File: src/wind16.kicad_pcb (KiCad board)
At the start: 2 copper layers, 78 x 78 mm, 49 parts, among them SW1 SW_Push_45deg, SW10 SW_Push_45deg, SW11 SW_Push_45deg, SW12 SW_Push_45deg, SW13 SW_Push_45deg, SW14 SW_Push_45deg, SW15 SW_Push_45deg, SW16 SW_Push_45deg, SW2 SW_Push_45deg, SW3 SW_Push_45deg, SW4 SW_Push_45deg, SW5 SW_Push_45deg, SW6 SW_Push_45deg, SW7 SW_Push_45deg, SW8 SW_Push_45deg, SW9 SW_Push_45deg, U1 MCU_Seeed_XIAO_RP2040

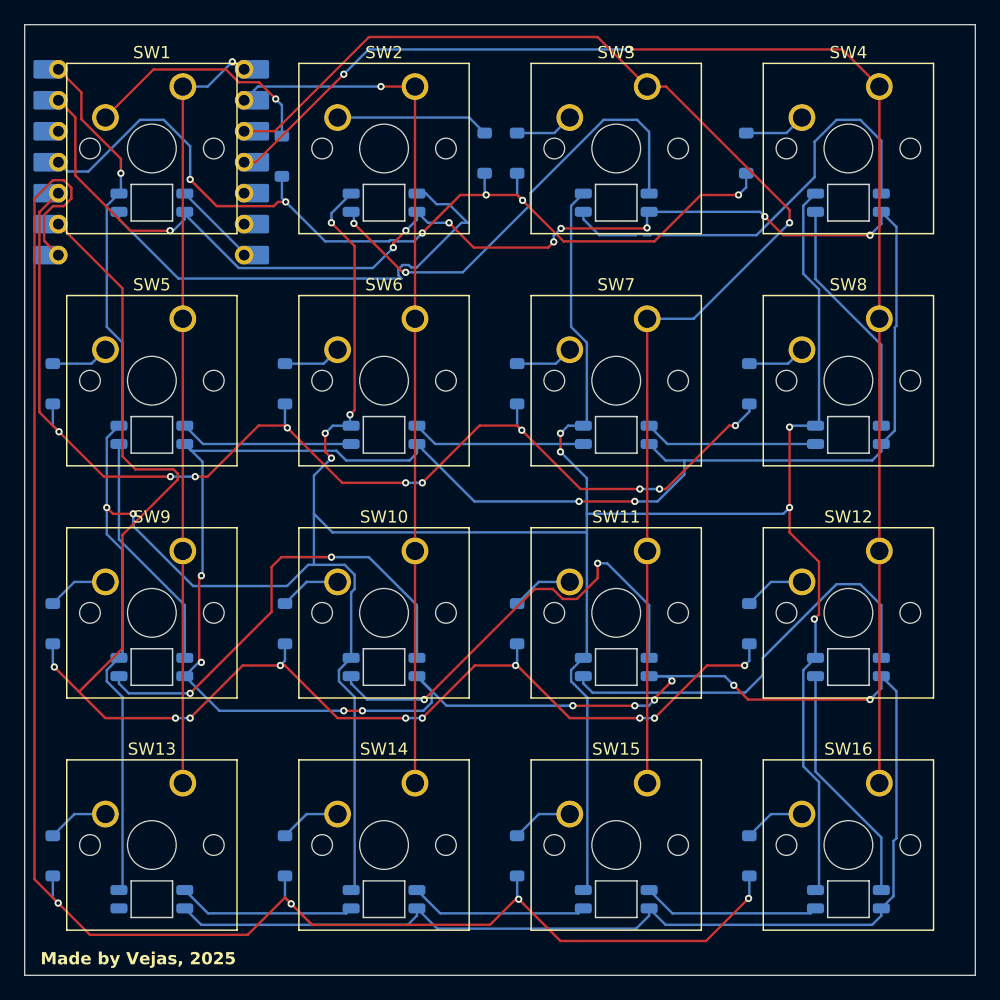
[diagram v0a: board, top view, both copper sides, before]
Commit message: loads of shit 1.3
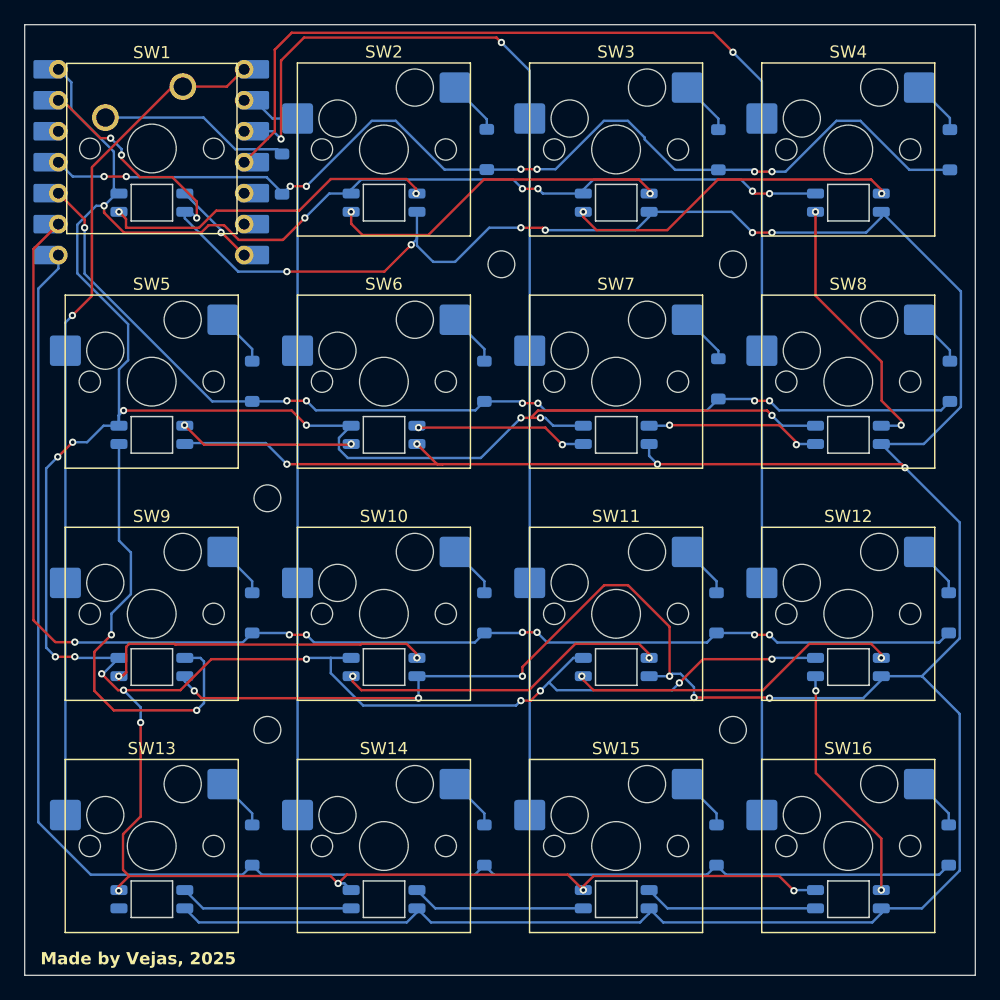
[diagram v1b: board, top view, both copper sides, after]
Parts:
- added REF**: MountingHole_2.2mm_M2, MountingHole:MountingHole_2.2mm_M2, F.Cu at (80.6, 66.8)
- added REF**: MountingHole_2.2mm_M2, MountingHole:MountingHole_2.2mm_M2, F.Cu at (99.8, 47.6)
- added REF**: MountingHole_2.2mm_M2, MountingHole:MountingHole_2.2mm_M2, F.Cu at (118.8, 47.6)
- added REF**: MountingHole_2.2mm_M2, MountingHole:MountingHole_2.2mm_M2, F.Cu at (80.6, 85.8)
- added REF**: MountingHole_2.2mm_M2, MountingHole:MountingHole_2.2mm_M2, F.Cu at (118.8, 85.8)
- SW10, SW11, SW12, SW13, SW14, SW15, SW16, SW2, SW3, SW4, SW5, SW6, SW7, SW8, SW9: footprint Button_Switch_Keyboard:SW_Cherry_MX_1.00u_PCB -> ScottoKeebs_Hotswap:Hotswap_MX_1.00u
- moved D4 16.7 mm to (136.6, 38.2)
- moved D7 16.5 mm to (117.6, 57.0)
- moved D3 16.5 mm to (117.6, 38.2)
- moved D8 16.5 mm to (136.6, 57.2)
- moved D10 16.4 mm to (98.4, 76.2)
- moved D11 16.4 mm to (117.5, 76.2)
- moved D12 16.4 mm to (136.5, 76.2)
- moved D14 16.4 mm to (98.4, 95.2)
- moved D15 16.4 mm to (117.5, 95.2)
- moved D16 16.4 mm to (136.5, 95.2)
- moved D13 16.4 mm to (79.3, 95.2)
- moved D9 16.4 mm to (79.3, 76.2)
- moved D6 16.4 mm to (98.4, 57.2)
- moved D5 16.4 mm to (79.3, 57.2)
- moved SW11 5.76 mm to (109.2, 76.3)
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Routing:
- net +5V: track 323.4 -> 347.1 mm, vias 12 -> 27
- net Net-(D24-DOUT): track 19.8 -> 36.9 mm, vias 0 -> 2
- net GND: track 345.9 -> 362.4 mm, vias 21 -> 19
- net r4: track 142.4 -> 126.0 mm, vias 4 -> 0
- net c3: track 107.9 -> 92.3 mm, vias 1 -> 2
- net r2: track 97.0 -> 84.9 mm, vias 10 -> 7
- net Net-(D17-DOUT): track 39.2 -> 27.8 mm, vias 0 -> 2
- net r3: track 122.6 -> 111.5 mm, vias 10 -> 7
- net c2: track 71.6 -> 61.3 mm, vias 1 -> 0
- net Net-(D25-DOUT): track 38.1 -> 27.9 mm
- net Net-(D26-DOUT): track 37.4 -> 27.4 mm
- net Net-(D18-DOUT): track 38.1 -> 28.5 mm
- net Net-(D19-DOUT): track 36.4 -> 27.8 mm, vias 0 -> 2
- net r1: track 77.2 -> 85.3 mm, vias 6 -> 8
- net Net-(D2-A): track 12.6 -> 4.51 mm
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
